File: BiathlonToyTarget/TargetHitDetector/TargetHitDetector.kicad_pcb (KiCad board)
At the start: 2 copper layers, 32 x 32 mm, 18 parts, among them J1 Screw_Terminal_01x03, U1 LM321, U2 LM321

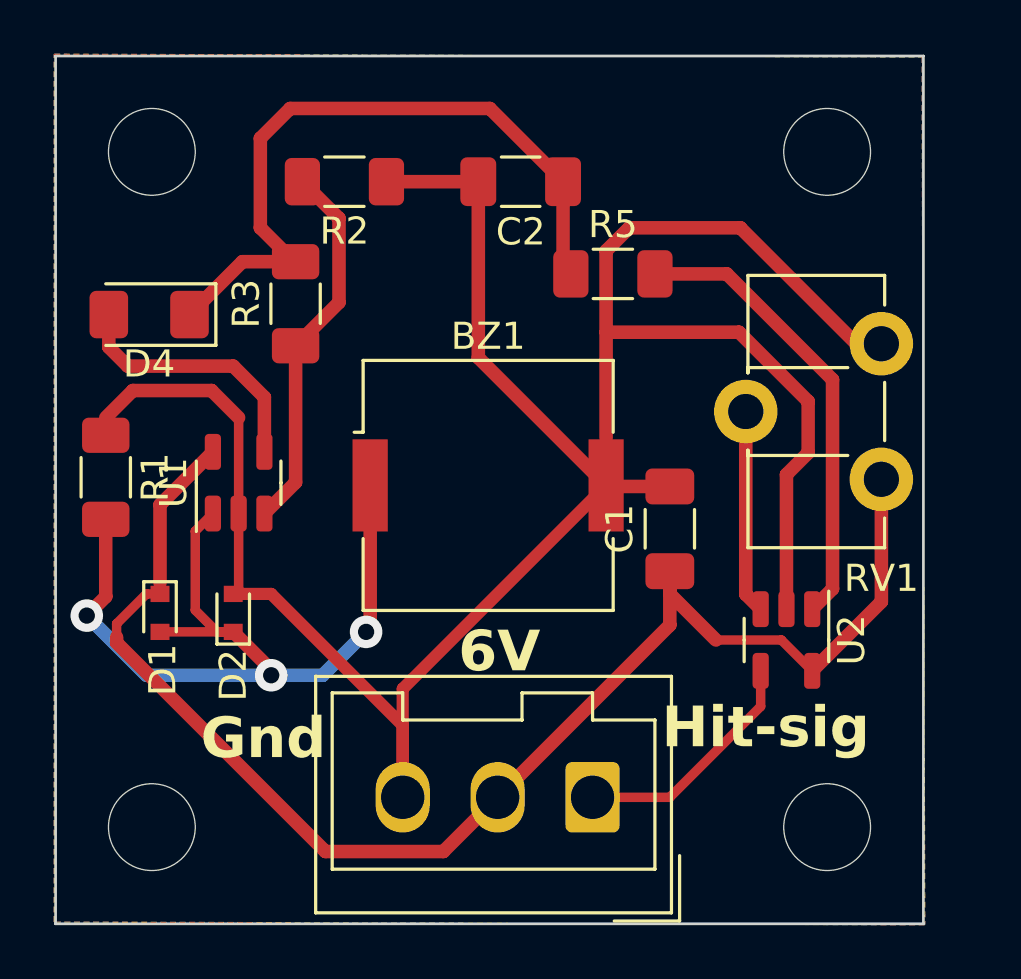
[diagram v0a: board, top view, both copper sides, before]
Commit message: Checking in the current design and prod files.
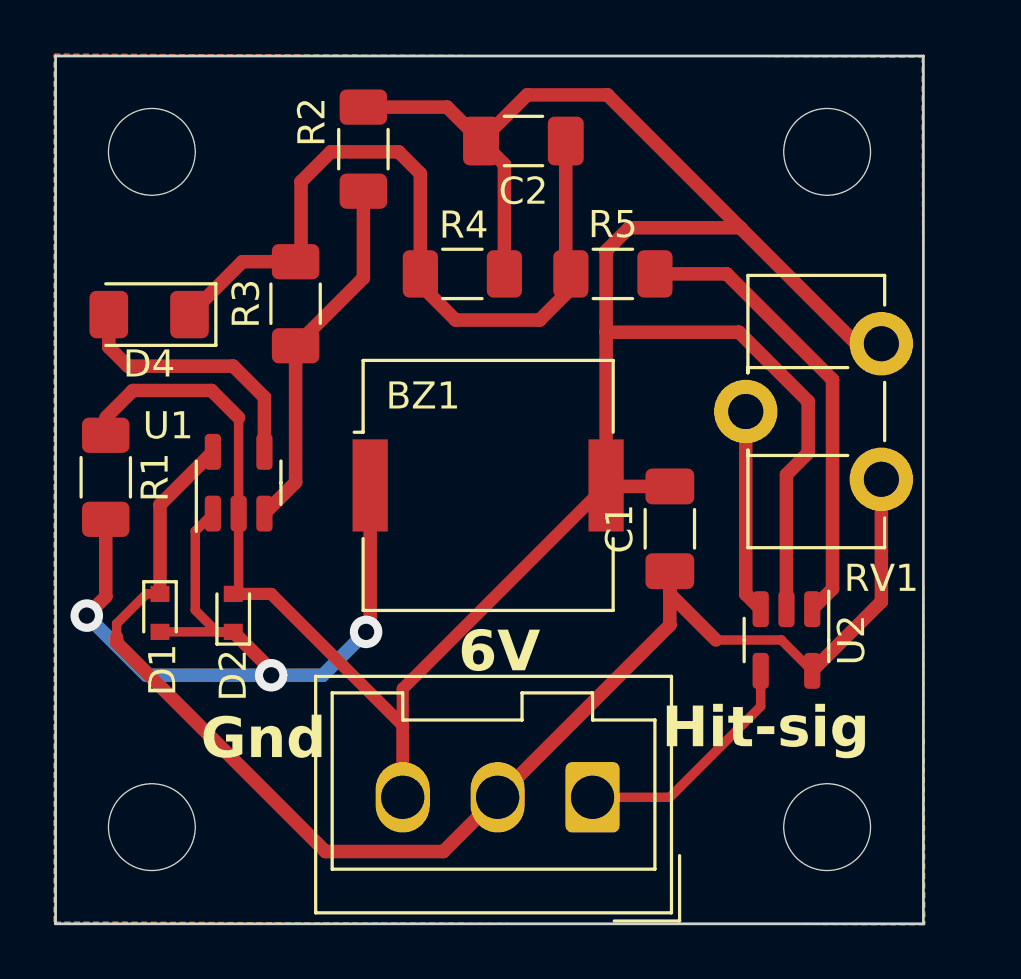
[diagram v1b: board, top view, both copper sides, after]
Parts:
- removed REF** (x4): MountingHole_3.2mm_M3, MountingHole:MountingHole_3.2mm_M3
- added H1: MountingHole, MountingHole:MountingHole_3.2mm_M3, F.Cu at (133.5, 86.6)
- added H2: MountingHole, MountingHole:MountingHole_3.2mm_M3, F.Cu at (158.4, 86.6)
- added H3: MountingHole, MountingHole:MountingHole_3.2mm_M3, F.Cu at (133.5, 111.5)
- added H4: MountingHole, MountingHole:MountingHole_3.2mm_M3, F.Cu at (158.4, 111.5)
- added R4: 1k, Resistor_SMD:R_1206_3216Metric_Pad1.30x1.75mm_HandSolder, F.Cu at (144.9, 91.1)
- C2: value 0.47u -> 1µF
- moved C2 1.50 mm to (147.2, 86.2)
- moved R2 1.39 mm to (141.3, 86.5), turned to -90 degrees
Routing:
- net Earth: track 96.6 -> 102.4 mm
- net Net-(D4-K): track 26.1 -> 29.6 mm
- net Net-(U1--): track 13.9 -> 13.4 mm
